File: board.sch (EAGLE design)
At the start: 2 parts

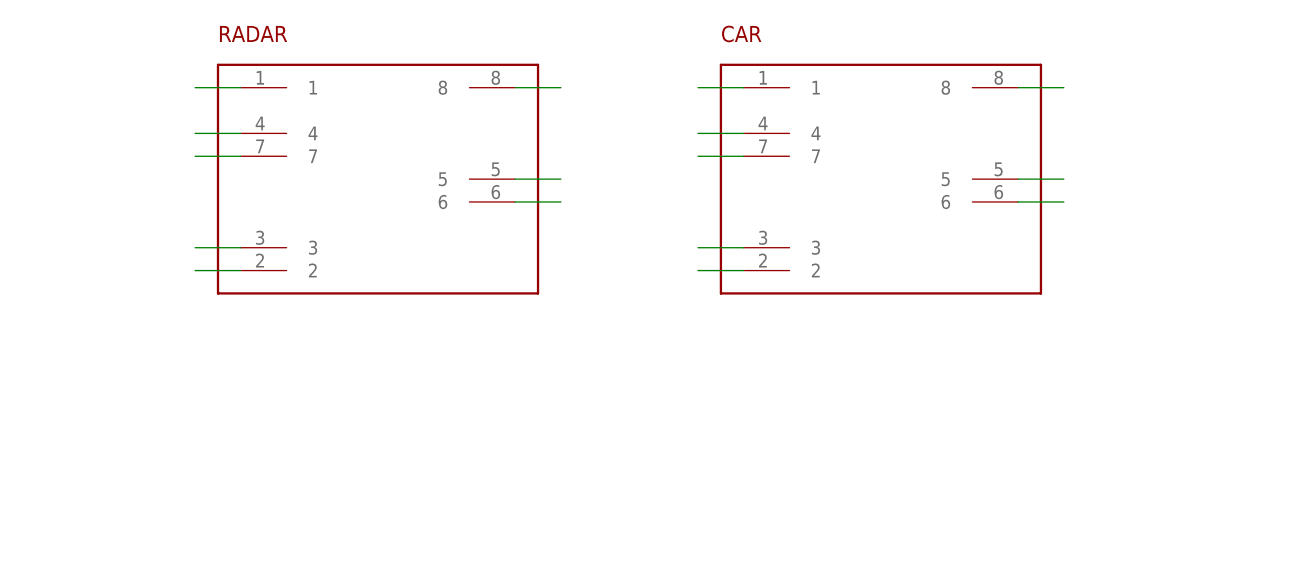
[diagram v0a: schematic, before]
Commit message: v0.2
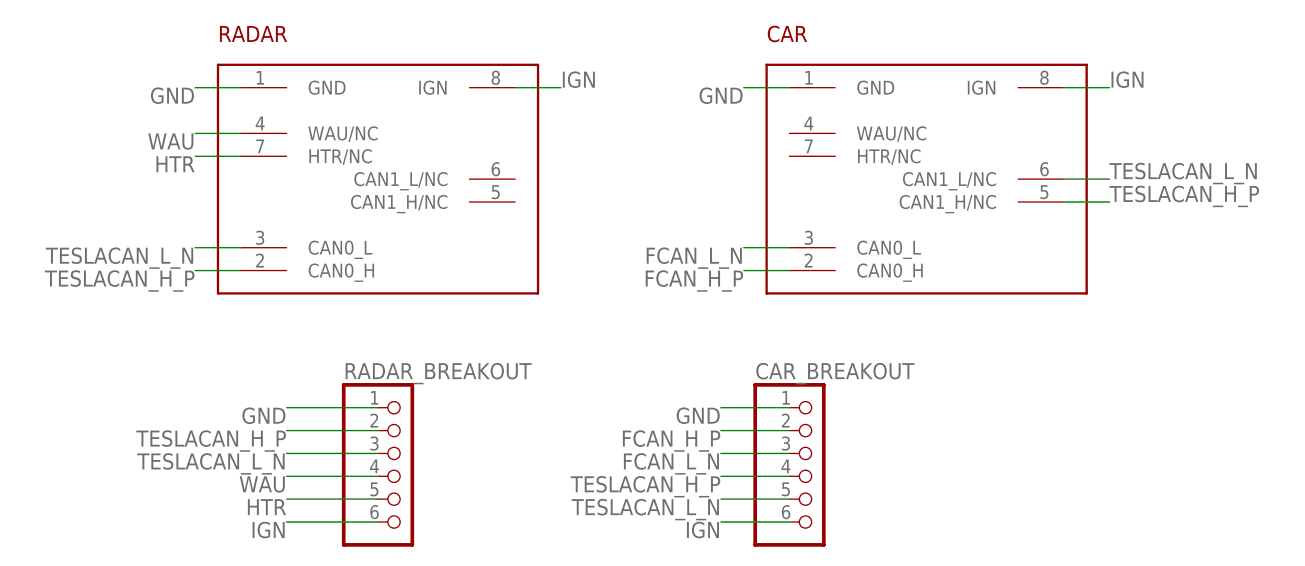
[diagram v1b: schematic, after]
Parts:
- added CAR_BREAKOUT, RADAR_BREAKOUT: (no value), pinhead:PINHD-1X6
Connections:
- removed net N$1: RADAR.1
- removed net N$10: CAR.8
- removed net N$11: CAR.5
- removed net N$12: CAR.6
- removed net N$13: CAR.4
- removed net N$14: CAR.7
- removed net N$15: RADAR.4
- removed net N$16: RADAR.7
- removed net N$2: RADAR.2
- removed net N$3: RADAR.3
- removed net N$4: RADAR.8
- removed net N$5: RADAR.5
- removed net N$6: RADAR.6
- removed net N$7: CAR.1
- removed net N$8: CAR.3
- removed net N$9: CAR.2
- new net FCAN_H_P: CAR.CAN0_H, CAR_BREAKOUT.2
- new net FCAN_L_N: CAR.CAN0_L, CAR_BREAKOUT.3
- new net GND: CAR.GND, CAR_BREAKOUT.1, RADAR.GND, RADAR_BREAKOUT.1
- new net HTR: RADAR.HTR/NC, RADAR_BREAKOUT.5
- new net IGN: CAR.IGN, CAR_BREAKOUT.6, RADAR.IGN, RADAR_BREAKOUT.6
- new net TESLACAN_H_P: CAR.CAN1_H/NC, CAR_BREAKOUT.4, RADAR.CAN0_H, RADAR_BREAKOUT.2
- new net TESLACAN_L_N: CAR.CAN1_L/NC, CAR_BREAKOUT.5, RADAR.CAN0_L, RADAR_BREAKOUT.3
- new net WAU: RADAR.WAU/NC, RADAR_BREAKOUT.4
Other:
- moved on the sheet: CAR
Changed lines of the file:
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@@
 <class number="0" name="default" width="0" drill="0">
+</class>
+<class number="1" name="diff pairs" width="0.3048" drill="0">
+<clearance class="1" value="0.254"/>
+</class>
+<class number="2" name="hipower" width="0.889" drill="0">
+</class>
+<class number="3" name="gnd" width="0.4064" drill="0">
 </class>
 </classes>
@@
 <part name="RADAR" library="Souers" deviceset="TE_AMP_1-1534229-1" device="TESLARADAR"/>
 <part name="CAR" library="Souers" deviceset="TE_AMP_1-967658-1" device=""/>
+<part name="CAR_BREAKOUT" library="pinhead" library_urn="urn:adsk.eagle:library:325" deviceset="PINHD-1X6" device="" package3d_urn="urn:adsk.eagle:package:22472/2"/>
+<part name="RADAR_BREAKOUT" library="pinhead" library_urn="urn:adsk.eagle:library:325" deviceset="PINHD-1X6" device="" package3d_urn="urn:adsk.eagle:package:22472/2"/>
 </parts>
 <sheets>
@@
 <instances>
 <instance part="RADAR" gate="G$1" x="17.78" y="43.18"/>
-<instance part="CAR" gate="G$1" x="73.66" y="43.18"/>
+<instance part="CAR" gate="G$1" x="78.74" y="43.18"/>
+<instance part="CAR_BREAKOUT" gate="A" x="68.58" y="12.7"/>
+<instance part="RADAR_BREAKOUT" gate="A" x="22.86" y="12.7"/>
 </instances>
 <busses>
 </busses>
 <nets>
-<net name="N$1" class="0">
+<net name="GND" class="3">
 <segment>
-<pinref part="RADAR" gate="G$1" pin="1"/>
+<pinref part="RADAR" gate="G$1" pin="GND"/>
 <wire x1="5.08" y1="55.88" x2="0" y2="55.88" width="0.1524" layer="91"/>
+<label x="0" y="55.88" size="1.778" layer="95" rot="R180"/>
+</segment>
+<segment>
+<pinref part="CAR" gate="G$1" pin="GND"/>
+<wire x1="66.04" y1="55.88" x2="60.96" y2="55.88" width="0.1524" layer="91"/>
+<label x="60.96" y="55.88" size="1.778" layer="95" rot="R180"/>
+</segment>
+<segment>
+<pinref part="RADAR_BREAKOUT" gate="A" pin="1"/>
+<wire x1="20.32" y1="20.32" x2="10.16" y2="20.32" width="0.1524" layer="91"/>
+<label x="10.16" y="20.32" size="1.778" layer="95" rot="R180"/>
+</segment>
+<segment>
+<pinref part="CAR_BREAKOUT" gate="A" pin="1"/>
+<wire x1="66.04" y1="20.32" x2="58.42" y2="20.32" width="0.1524" layer="91"/>
+<label x="58.42" y="20.32" size="1.778" layer="95" rot="R180"/>
 </segment>
 </net>
-<net name="N$2" class="0">
+<net name="TESLACAN_H_P" class="1">
 <segment>
-<pinref part="RADAR" gate="G$1" pin="2"/>
+<pinref part="RADAR" gate="G$1" pin="CAN0_H"/>
 <wire x1="5.08" y1="35.56" x2="0" y2="35.56" width="0.1524" layer="91"/>
+<label x="0" y="35.56" size="1.778" layer="95" rot="R180"/>
+</segment>
+<segment>
+<pinref part="RADAR_BREAKOUT" gate="A" pin="2"/>
+<wire x1="20.32" y1="17.78" x2="10.16" y2="17.78" width="0.1524" layer="91"/>
+<label x="10.16" y="17.78" size="1.778" layer="95" rot="R180"/>
+</segment>
+<segment>
+<pinref part="CAR_BREAKOUT" gate="A" pin="4"/>
+<wire x1="66.04" y1="12.7" x2="58.42" y2="12.7" width="0.1524" layer="91"/>
+<label x="58.42" y="12.7" size="1.778" layer="95" rot="R180"/>
+</segment>
+<segment>
+<pinref part="CAR" gate="G$1" pin="CAN1_H/NC"/>
+<wire x1="96.52" y1="43.18" x2="101.6" y2="43.18" width="0.1524" layer="91"/>
+<label x="101.6" y="43.18" size="1.778" layer="95"/>
 </segment>
 </net>
-<net name="N$3" class="0">
+<net name="TESLACAN_L_N" class="1">
 <segment>
-<pinref part="RADAR" gate="G$1" pin="3"/>
+<pinref part="RADAR_BREAKOUT" gate="A" pin="3"/>
+<wire x1="20.32" y1="15.24" x2="10.16" y2="15.24" width="0.1524" layer="91"/>
+<label x="10.16" y="15.24" size="1.778" layer="95" rot="R180"/>
+</segment>
+<segment>
+<pinref part="CAR_BREAKOUT" gate="A" pin="5"/>
+<wire x1="66.04" y1="10.16" x2="58.42" y2="10.16" width="0.1524" layer="91"/>
+<label x="58.42" y="10.16" size="1.778" layer="95" rot="R180"/>
+</segment>
+<segment>
+<pinref part="RADAR" gate="G$1" pin="CAN0_L"/>
 <wire x1="5.08" y1="38.1" x2="0" y2="38.1" width="0.1524" layer="91"/>
+<label x="0" y="38.1" size="1.778" layer="95" rot="R180"/>
+</segment>
+<segment>
+<pinref part="CAR" gate="G$1" pin="CAN1_L/NC"/>
+<wire x1="96.52" y1="45.72" x2="101.6" y2="45.72" width="0.1524" layer="91"/>
+<label x="101.6" y="45.72" size="1.778" layer="95"/>
 </segment>
 </net>
-<net name="N$4" class="0">
+<net name="FCAN_L_N" class="1">
 <segment>
-<pinref part="RADAR" gate="G$1" pin="8"/>
-<wire x1="35.56" y1="55.88" x2="40.64" y2="55.88" width="0.1524" layer="91"/>
+<pinref part="CAR" gate="G$1" pin="CAN0_L"/>
+<wire x1="66.04" y1="38.1" x2="60.96" y2="38.1" width="0.1524" layer="91"/>
+<label x="60.96" y="38.1" size="1.778" layer="95" rot="R180"/>
+</segment>
+<segment>
+<pinref part="CAR_BREAKOUT" gate="A" pin="3"/>
+<wire x1="66.04" y1="15.24" x2="58.42" y2="15.24" width="0.1524" layer="91"/>
+<label x="58.42" y="15.24" size="1.778" layer="95" rot="R180"/>
 </segment>
 </net>
-<net name="N$5" class="0">
+<net name="FCAN_H_P" class="1">
 <segment>
-<pinref part="RADAR" gate="G$1" pin="5"/>
-<wire x1="35.56" y1="45.72" x2="40.64" y2="45.72" width="0.1524" layer="91"/>
+<pinref part="CAR" gate="G$1" pin="CAN0_H"/>
+<wire x1="66.04" y1="35.56" x2="60.96" y2="35.56" width="0.1524" layer="91"/>
+<label x="60.96" y="35.56" size="1.778" layer="95" rot="R180"/>
+</segment>
+<segment>
+<pinref part="CAR_BREAKOUT" gate="A" pin="2"/>
+<wire x1="66.04" y1="17.78" x2="58.42" y2="17.78" width="0.1524" layer="91"/>
+<label x="58.42" y="17.78" size="1.778" layer="95" rot="R180"/>
 </segment>
 </net>
-<net name="N$6" class="0">
+<net name="HTR" class="2">
 <segment>
-<pinref part="RADAR" gate="G$1" pin="6"/>
-<wire x1="35.56" y1="43.18" x2="40.64" y2="43.18" width="0.1524" layer="91"/>
+<pinref part="RADAR" gate="G$1" pin="HTR/NC"/>
+<wire x1="5.08" y1="48.26" x2="0" y2="48.26" width="0.1524" layer="91"/>
+<label x="0" y="48.26" size="1.778" layer="95" rot="R180"/>
+</segment>
+<segment>
+<pinref part="RADAR_BREAKOUT" gate="A" pin="5"/>
+<wire x1="20.32" y1="10.16" x2="10.16" y2="10.16" width="0.1524" layer="91"/>
+<label x="10.16" y="10.16" size="1.778" layer="95" rot="R180"/>
 </segment>
 </net>
-<net name="N$7" class="0">
+<net name="IGN" class="2">
 <segment>
-<pinref part="CAR" gate="G$1" pin="1"/>
-<wire x1="60.96" y1="55.88" x2="55.88" y2="55.88" width="0.1524" layer="91"/>
+<pinref part="RADAR" gate="G$1" pin="IGN"/>
+<wire x1="35.56" y1="55.88" x2="40.64" y2="55.88" width="0.1524" layer="91"/>
+<label x="40.64" y="55.88" size="1.778" layer="95"/>
+</segment>
+<segment>
+<pinref part="CAR" gate="G$1" pin="IGN"/>
+<wire x1="96.52" y1="55.88" x2="101.6" y2="55.88" width="0.1524" layer="91"/>
+<label x="101.6" y="55.88" size="1.778" layer="95"/>
+</segment>
+<segment>
+<pinref part="RADAR_BREAKOUT" gate="A" pin="6"/>
+<wire x1="20.32" y1="7.62" x2="10.16" y2="7.62" width="0.1524" layer="91"/>
+<label x="10.16" y="7.62" size="1.778" layer="95" rot="R180"/>
+</segment>
+<segment>
+<pinref part="CAR_BREAKOUT" gate="A" pin="6"/>
+<wire x1="66.04" y1="7.62" x2="58.42" y2="7.62" width="0.1524" layer="91"/>
+<label x="58.42" y="7.62" size="1.778" layer="95" rot="R180"/>
 </segment>
 </net>
-<net name="N$8" class="0">
+<net name="WAU" class="0">
 <segment>
-<pinref part="CAR" gate="G$1" pin="3"/>
-<wire x1="60.96" y1="38.1" x2="55.88" y2="38.1" width="0.1524" layer="91"/>
+<pinref part="RADAR_BREAKOUT" gate="A" pin="4"/>
+<wire x1="20.32" y1="12.7" x2="10.16" y2="12.7" width="0.1524" layer="91"/>
+<label x="10.16" y="12.7" size="1.778" layer="95" rot="R180"/>
 </segment>
-</net>
-<net name="N$9" class="0">
 <segment>
-<pinref part="CAR" gate="G$1" pin="2"/>
-<wire x1="60.96" y1="35.56" x2="55.88" y2="35.56" width="0.1524" layer="91"/>
-</segment>
-</net>
-<net name="N$10" class="0">
-<segment>
-<pinref part="CAR" gate="G$1" pin="8"/>
-<wire x1="91.44" y1="55.88" x2="96.52" y2="55.88" width="0.1524" layer="91"/>
-</segment>
-</net>
-<net name="N$11" class="0">
-<segment>
-<pinref part="CAR" gate="G$1" pin="5"/>
-<wire x1="91.44" y1="45.72" x2="96.52" y2="45.72" width="0.1524" layer="91"/>
-</segment>
-</net>
-<net name="N$12" class="0">
-<segment>
-<pinref part="CAR" gate="G$1" pin="6"/>
-<wire x1="91.44" y1="43.18" x2="96.52" y2="43.18" width="0.1524" layer="91"/>
-</segment>
-</net>
-<net name="N$13" class="0">
-<segment>
-<pinref part="CAR" gate="G$1" pin="4"/>
-<wire x1="60.96" y1="50.8" x2="55.88" y2="50.8" width="0.1524" layer="91"/>
-</segment>
-</net>
-<net name="N$14" class="0">
-<segment>
-<pinref part="CAR" gate="G$1" pin="7"/>
-<wire x1="60.96" y1="48.26" x2="55.88" y2="48.26" width="0.1524" layer="91"/>
-</segment>
-</net>
-<net name="N$15" class="0">
-<segment>
-<pinref part="RADAR" gate="G$1" pin="4"/>
+<pinref part="RADAR" gate="G$1" pin="WAU/NC"/>
 <wire x1="5.08" y1="50.8" x2="0" y2="50.8" width="0.1524" layer="91"/>
-</segment>
-</net>
-<net name="N$16" class="0">
-<segment>
-<pinref part="RADAR" gate="G$1" pin="7"/>
-<wire x1="5.08" y1="48.26" x2="0" y2="48.26" width="0.1524" layer="91"/>
+<label x="0" y="50.8" size="1.778" layer="95" rot="R180"/>
 </segment>
 </net>
@@
 </sheet>
 </sheets>
+<errors>
+</errors>
 </schematic>
 </drawing>
+<compatibility>
+<note version="8.2" severity="warning">
+Since Version 8.2, EAGLE supports online libraries. The ids
+of those online libraries will not be understood (or retained)
+with this version.
+</note>
+<note version="8.3" severity="warning">
+Since Version 8.3, EAGLE supports URNs for individual library
+assets (packages, symbols, and devices). The URNs of those assets
+will not be understood (or retained) with this version.
+</note>
+<note version="8.3" severity="warning">
+Since Version 8.3, EAGLE supports the association of 3D packages
+with devices in libraries, schematics, and board files. Those 3D
+packages will not be understood (or retained) with this version.
+</note>
+</compatibility>
 </eagle>
